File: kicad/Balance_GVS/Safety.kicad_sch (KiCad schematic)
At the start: 36 parts, among them J1 Conn_01x02_Pin, J16 Conn_01x01_Pin, J17 Conn_01x01_Pin, J6 Conn_01x03_Pin, J7 Conn_01x03_Pin, J8 Conn_01x05_Pin, K1 AQY210S, SW2 EVQ-P7A01P, U2 SN74LVC1G74DCUR, U3 OPA4313IPWR, U4 INA303A1IPW

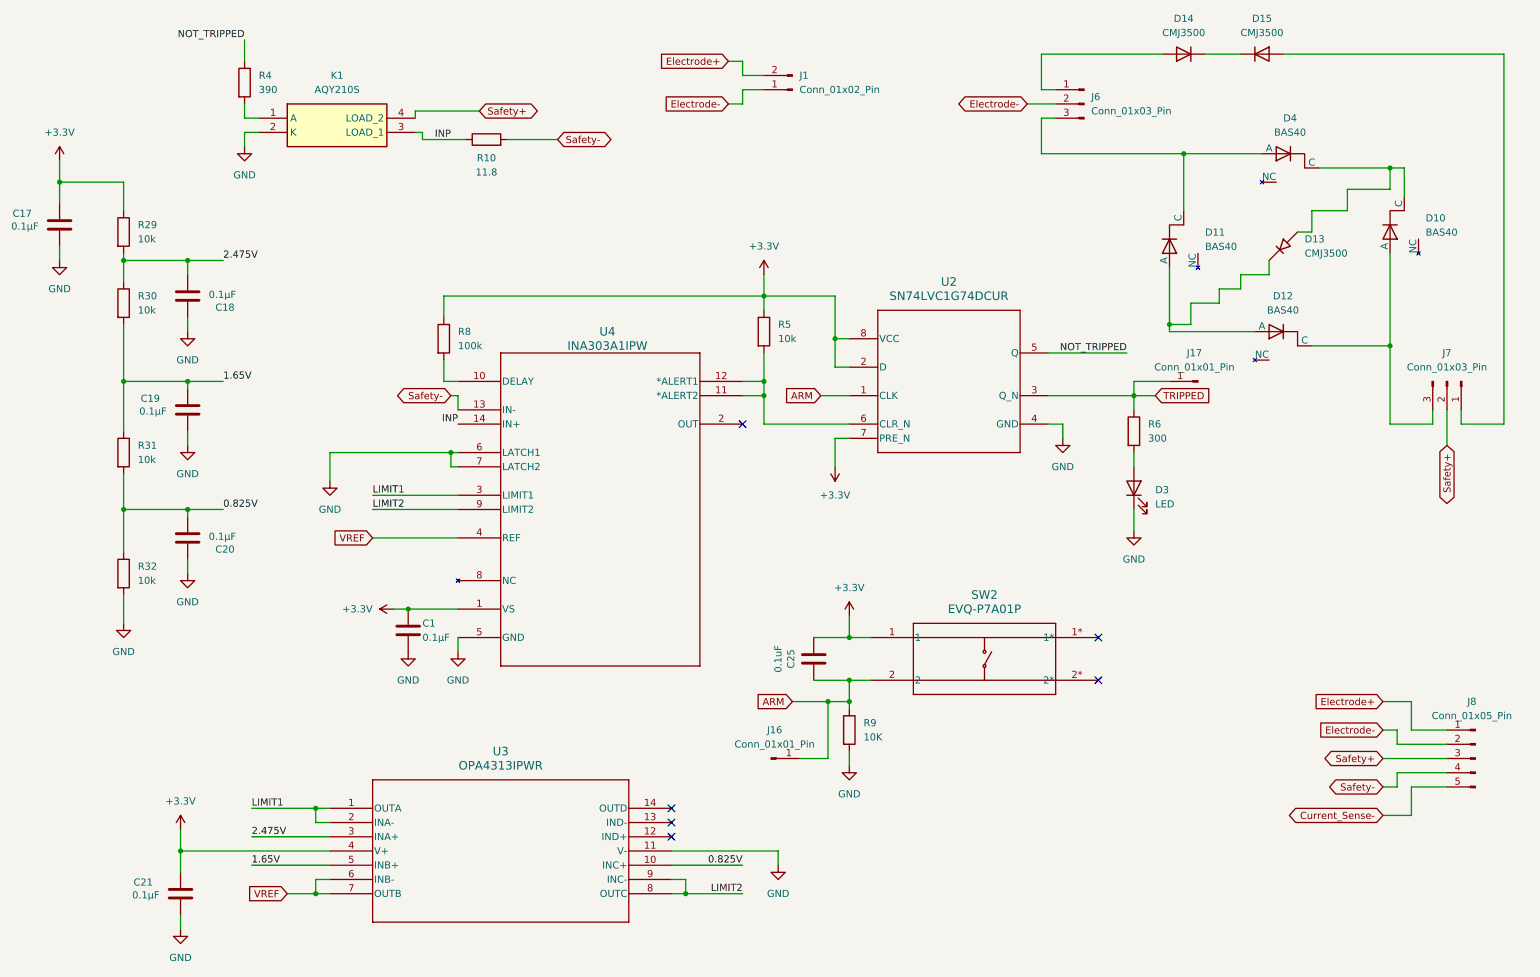
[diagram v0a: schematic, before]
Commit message: Add Mark debug point testing and udpate silkscreen
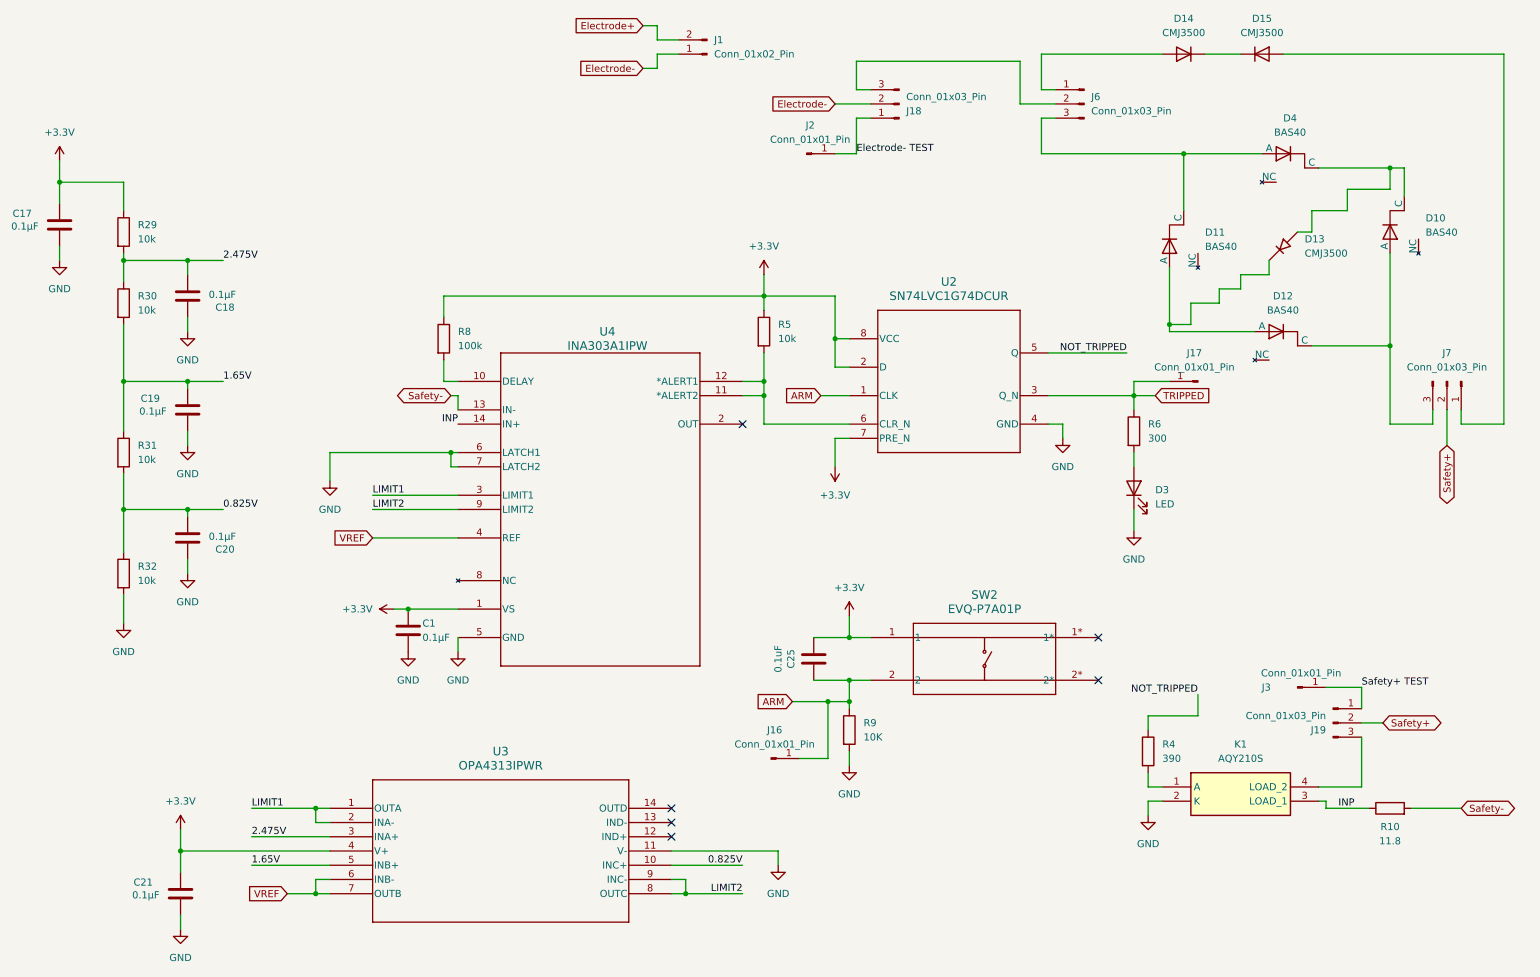
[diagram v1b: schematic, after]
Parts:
- removed J8: Conn_01x05_Pin, Connector_PinSocket_2.54mm:PinSocket_1x05_P2.54mm_Vertical, symbol Connector:Conn_01x05_Pin
- added J18, J19: Conn_01x03_Pin, Connector_PinHeader_2.54mm:PinHeader_1x03_P2.54mm_Vertical, symbol Connector:Conn_01x03_Pin
- added J2, J3: Conn_01x01_Pin, Connector_PinSocket_2.54mm:PinSocket_1x01_P2.54mm_Vertical, symbol Connector:Conn_01x01_Pin
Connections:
- net Electrode-: now also J18.2 (Pin_2); no longer J6.2 (Pin_2)
- net Safety+: now also J19.2 (Pin_2); no longer K1.4 (LOAD_2)
- new net: J19.3 (Pin_3), K1.4 (LOAD_2)
- new net: J18.3 (Pin_3), J6.2 (Pin_2)
- new net Electrode- TEST: J18.1 (Pin_1), J2.1 (Pin_1)
- new net Safety+ TEST: J19.1 (Pin_1), J3.1 (Pin_1)
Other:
- moved on the sheet: J1, K1, R10, R4
